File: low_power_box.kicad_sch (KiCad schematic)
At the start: 8 parts

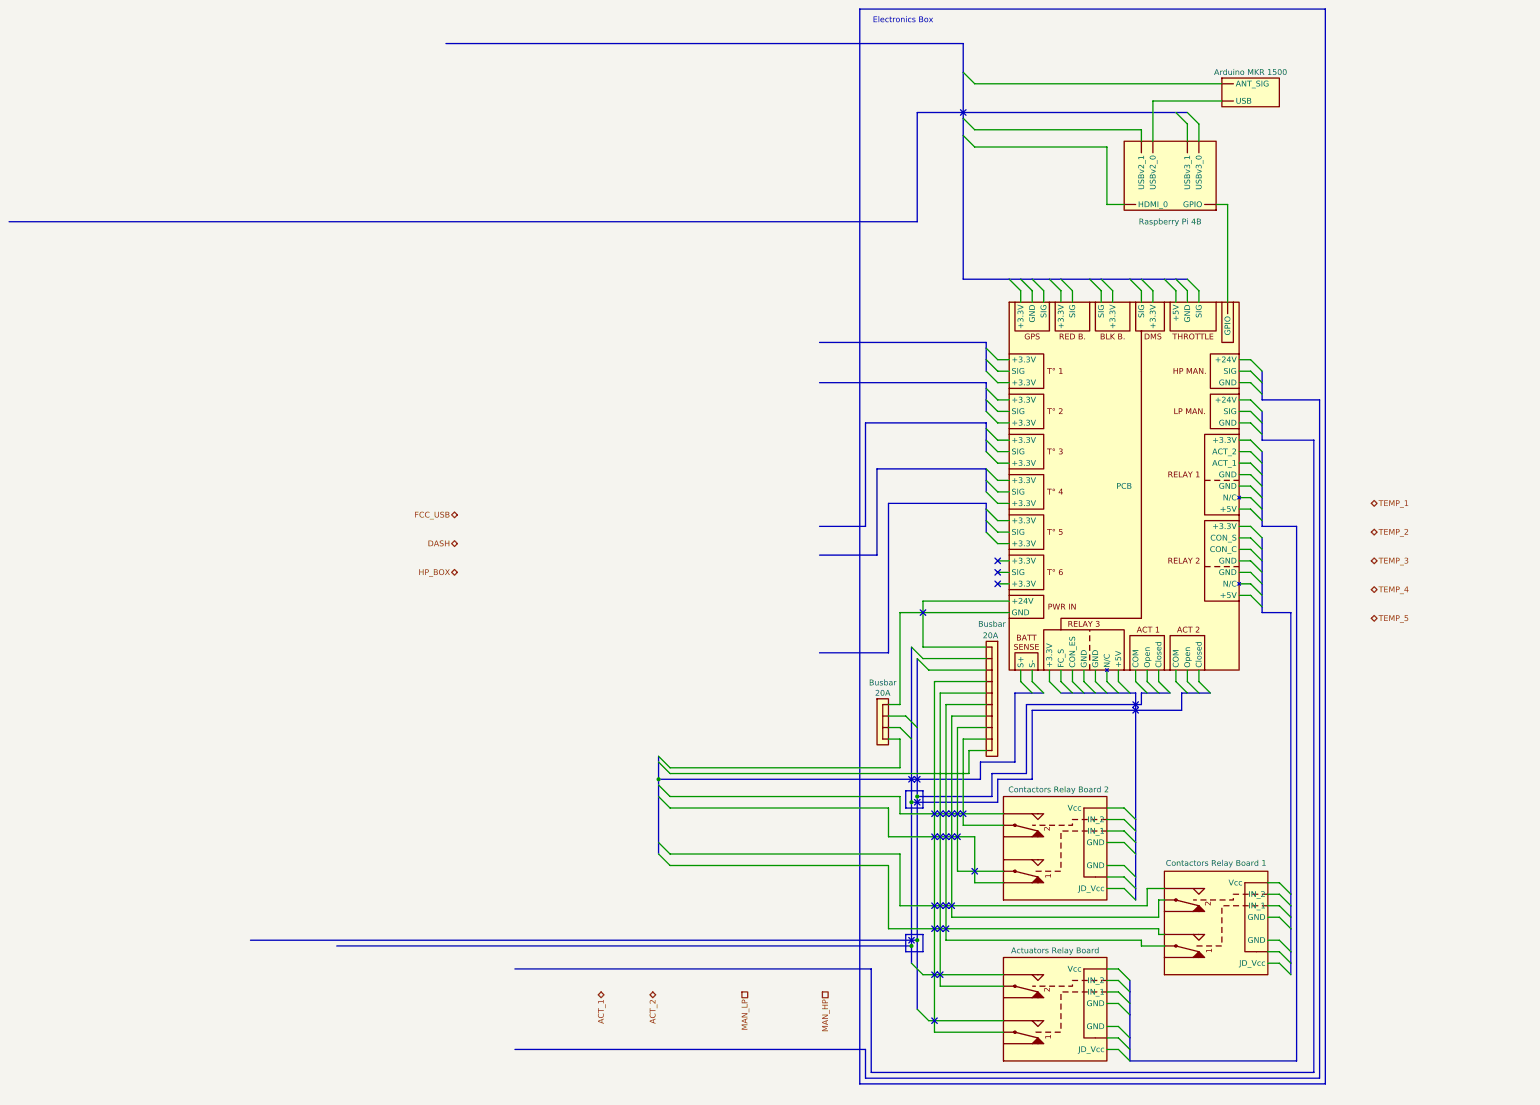
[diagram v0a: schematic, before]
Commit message: Complete Low Power Box
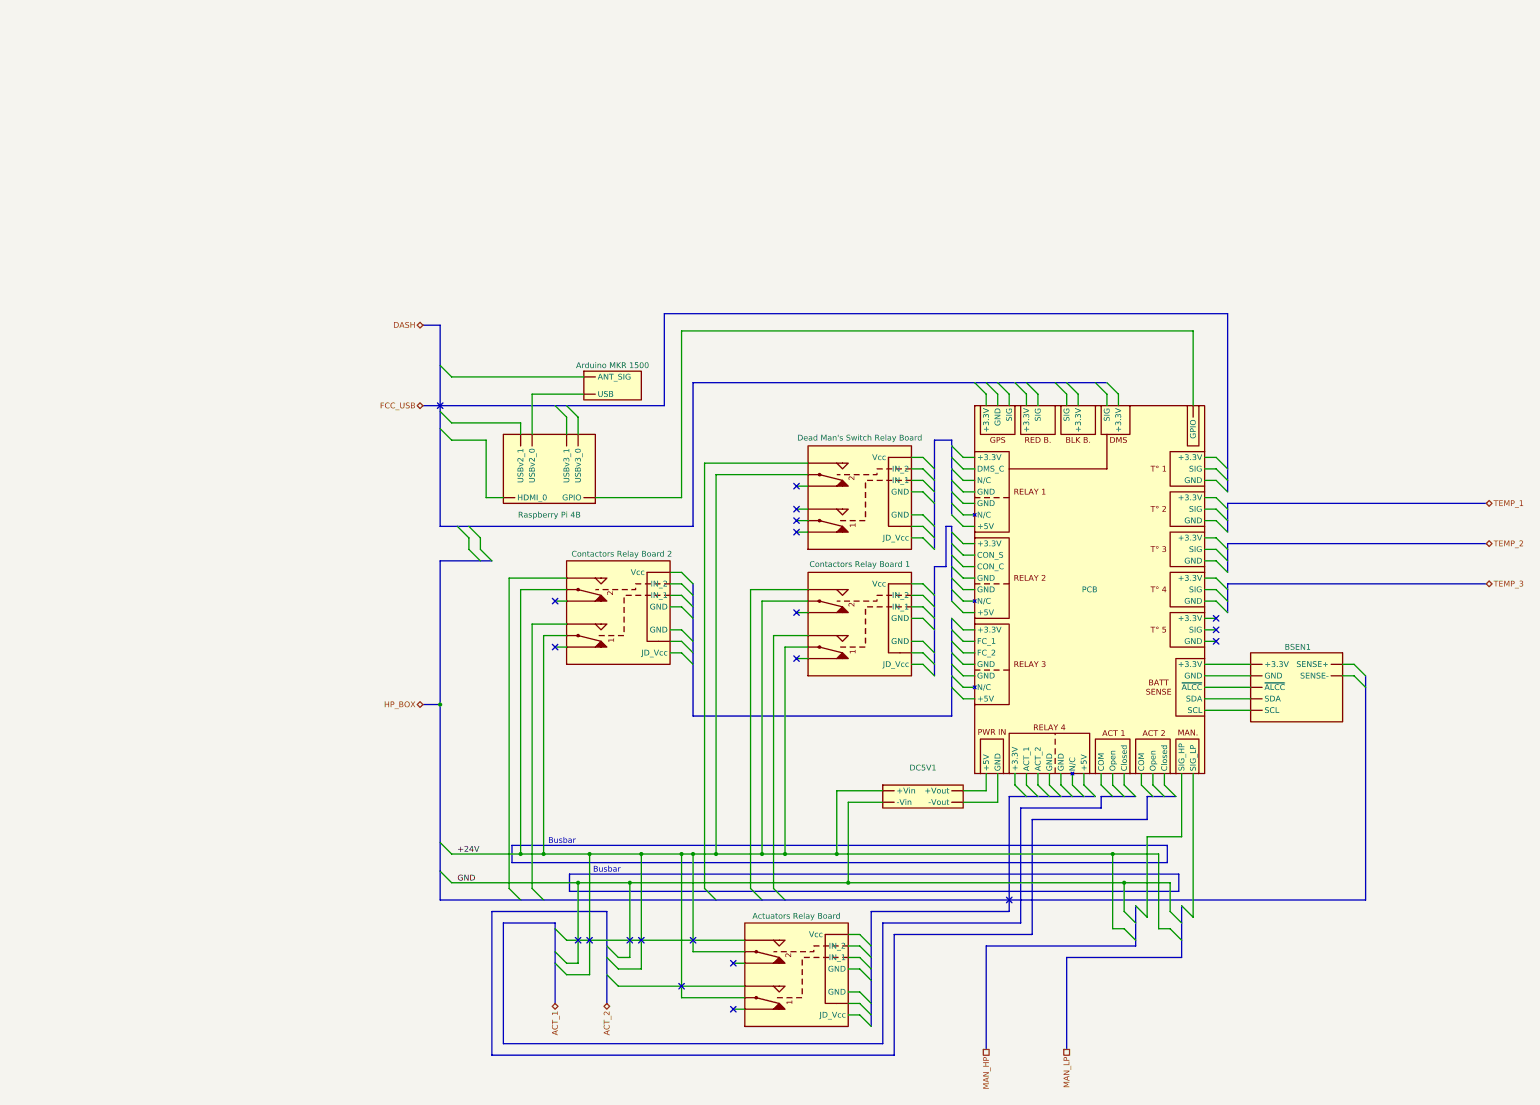
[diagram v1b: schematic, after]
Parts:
- removed BSB1: 20A, symbol Exocet_Electrical:Busbar_4
- removed BSB2: 20A, symbol Exocet_Electrical:Busbar_10
- added BSEN1: ~, symbol Exocet_Electrical:Battery_Sense
- added DC5V1: ~, symbol Exocet_Electrical:DC-DC_24V_5V
- added RELB4: ~, symbol Exocet_Electrical:Relay_Board
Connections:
- net +24V: now reaches RELB1. (Vcc)
- net +24V: now also RELB2. (Vcc), RELB3. (Vcc), DC5V1. (-Vout), RELB4. (Vcc)
- net at RPI1. (USBv3_1): now also ARD1. (USB); no longer PCB1. (SIG)
- net at ARD1. (USB): no longer RPI1. (USBv3_1)
- new net: BSEN1. (~{ALCC}), PCB1. (~{ALCC}) (x5)
- new net: DC5V1. (-Vout), PCB1. (~{ALCC}) (x2)
- new net: PCB1. (~{ALCC}), RPI1. (USBv3_1)
- new net GND: DC5V1. (-Vout)
- now unconnected: PCB1. (SIG)
- no-connect marks 33 -> 21
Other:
- note added: "Busbar"
- note removed: "Electronics Box"
